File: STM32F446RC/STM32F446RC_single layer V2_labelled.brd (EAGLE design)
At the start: 80.2 x 29 mm, 75 parts, among them IC1 STM32F446RCT6

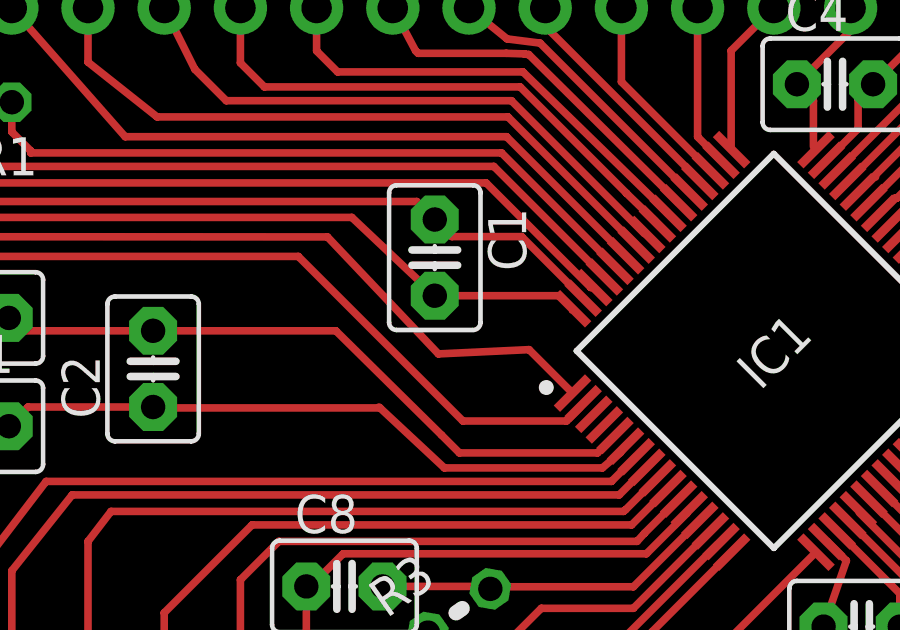
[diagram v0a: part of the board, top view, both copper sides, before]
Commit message: added final
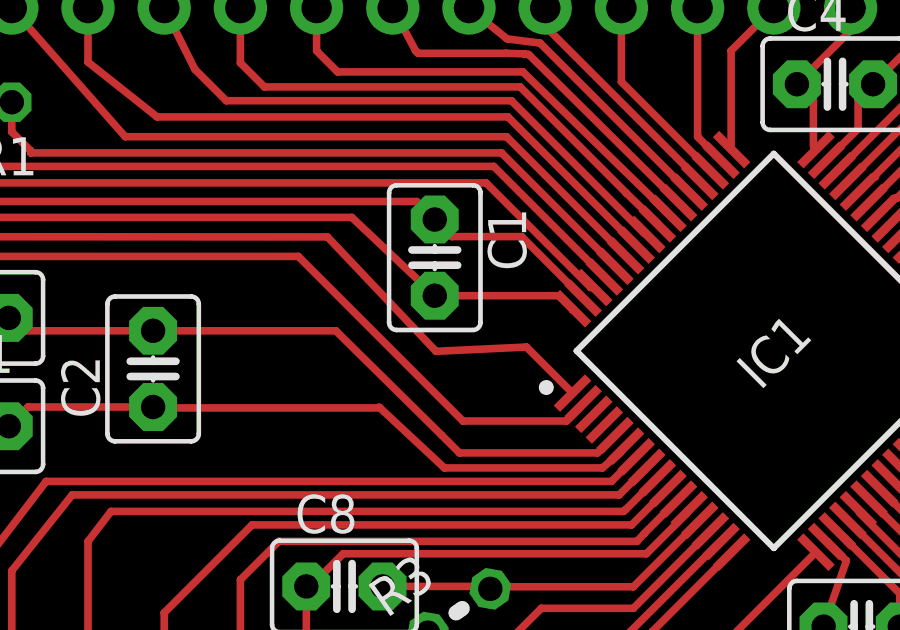
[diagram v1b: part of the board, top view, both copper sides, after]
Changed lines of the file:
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@@
 <layer number="16" name="Bottom" color="1" fill="1" visible="yes" active="yes"/>
 <layer number="17" name="Pads" color="2" fill="1" visible="yes" active="yes"/>
-<layer number="18" name="Vias" color="2" fill="1" visible="no" active="yes"/>
+<layer number="18" name="Vias" color="2" fill="1" visible="yes" active="yes"/>
 <layer number="19" name="Unrouted" color="6" fill="1" visible="yes" active="yes"/>
 <layer number="20" name="Dimension" color="24" fill="1" visible="yes" active="yes"/>
 <layer number="21" name="tPlace" color="7" fill="1" visible="yes" active="yes"/>
-<layer number="22" name="bPlace" color="7" fill="1" visible="no" active="yes"/>
+<layer number="22" name="bPlace" color="7" fill="1" visible="yes" active="yes"/>
 <layer number="23" name="tOrigins" color="15" fill="1" visible="yes" active="yes"/>
-<layer number="24" name="bOrigins" color="15" fill="1" visible="no" active="yes"/>
-<layer number="25" name="tNames" color="7" fill="1" visible="no" active="yes"/>
-<layer number="26" name="bNames" color="7" fill="1" visible="no" active="yes"/>
-<layer number="27" name="tValues" color="7" fill="1" visible="no" active="yes"/>
-<layer number="28" name="bValues" color="7" fill="1" visible="no" active="yes"/>
-<layer number="29" name="tStop" color="7" fill="3" visible="no" active="yes"/>
+<layer number="24" name="bOrigins" color="15" fill="1" visible="yes" active="yes"/>
+<layer number="25" name="tNames" color="7" fill="1" visible="yes" active="yes"/>
+<layer number="26" name="bNames" color="7" fill="1" visible="yes" active="yes"/>
+<layer number="27" name="tValues" color="7" fill="1" visible="yes" active="yes"/>
+<layer number="28" name="bValues" color="7" fill="1" visible="yes" active="yes"/>
+<layer number="29" name="tStop" color="7" fill="3" visible="yes" active="yes"/>
 <layer number="30" name="bStop" color="7" fill="6" visible="no" active="yes"/>
-<layer number="31" name="tCream" color="7" fill="4" visible="no" active="yes"/>
-<layer number="32" name="bCream" color="7" fill="5" visible="no" active="yes"/>
-<layer number="33" name="tFinish" color="6" fill="3" visible="no" active="yes"/>
-<layer number="34" name="bFinish" color="6" fill="6" visible="no" active="yes"/>
-<layer number="35" name="tGlue" color="7" fill="4" visible="no" active="yes"/>
-<layer number="36" name="bGlue" color="7" fill="5" visible="no" active="yes"/>
-<layer number="37" name="tTest" color="7" fill="1" visible="no" active="yes"/>
-<layer number="38" name="bTest" color="7" fill="1" visible="no" active="yes"/>
-<layer number="39" name="tKeepout" color="4" fill="11" visible="no" active="yes"/>
-<layer number="40" name="bKeepout" color="1" fill="11" visible="no" active="yes"/>
-<layer number="41" name="tRestrict" color="4" fill="10" visible="no" active="yes"/>
-<layer number="42" name="bRestrict" color="1" fill="10" visible="no" active="yes"/>
-<layer number="43" name="vRestrict" color="2" fill="10" visible="no" active="yes"/>
-<layer number="44" name="Drills" color="7" fill="1" visible="no" active="yes"/>
-<layer number="45" name="Holes" color="7" fill="1" visible="no" active="yes"/>
-<layer number="46" name="Milling" color="3" fill="1" visible="no" active="yes"/>
-<layer number="47" name="Measures" color="7" fill="1" visible="no" active="yes"/>
+<layer number="31" name="tCream" color="7" fill="4" visible="yes" active="yes"/>
+<layer number="32" name="bCream" color="7" fill="5" visible="yes" active="yes"/>
+<layer number="33" name="tFinish" color="6" fill="3" visible="yes" active="yes"/>
+<layer number="34" name="bFinish" color="6" fill="6" visible="yes" active="yes"/>
+<layer number="35" name="tGlue" color="7" fill="4" visible="yes" active="yes"/>
+<layer number="36" name="bGlue" color="7" fill="5" visible="yes" active="yes"/>
+<layer number="37" name="tTest" color="7" fill="1" visible="yes" active="yes"/>
+<layer number="38" name="bTest" color="7" fill="1" visible="yes" active="yes"/>
+<layer number="39" name="tKeepout" color="4" fill="11" visible="yes" active="yes"/>
+<layer number="40" name="bKeepout" color="1" fill="11" visible="yes" active="yes"/>
+<layer number="41" name="tRestrict" color="4" fill="10" visible="yes" active="yes"/>
+<layer number="42" name="bRestrict" color="1" fill="10" visible="yes" active="yes"/>
+<layer number="43" name="vRestrict" color="2" fill="10" visible="yes" active="yes"/>
+<layer number="44" name="Drills" color="7" fill="1" visible="yes" active="yes"/>
+<layer number="45" name="Holes" color="7" fill="1" visible="yes" active="yes"/>
+<layer number="46" name="Milling" color="3" fill="1" visible="yes" active="yes"/>
+<layer number="47" name="Measures" color="7" fill="1" visible="yes" active="yes"/>
 <layer number="48" name="Document" color="7" fill="1" visible="yes" active="yes"/>
-<layer number="49" name="Reference" color="7" fill="1" visible="no" active="yes"/>
+<layer number="49" name="Reference" color="7" fill="1" visible="yes" active="yes"/>
 <layer number="50" name="dxf" color="7" fill="1" visible="no" active="no"/>
-<layer number="51" name="tDocu" color="7" fill="1" visible="no" active="yes"/>
+<layer number="51" name="tDocu" color="7" fill="1" visible="yes" active="yes"/>
 <layer number="52" name="bDocu" color="7" fill="1" visible="yes" active="yes"/>
 <layer number="53" name="tGND_GNDA" color="7" fill="1" visible="no" active="no"/>
@@
 <layer number="221" name="221bmp" color="7" fill="1" visible="yes" active="yes"/>
 <layer number="222" name="222bmp" color="7" fill="1" visible="yes" active="yes"/>
-<layer number="223" name="223bmp" color="7" fill="1" visible="no" active="yes"/>
-<layer number="224" name="224bmp" color="7" fill="1" visible="no" active="yes"/>
-<layer number="250" name="Descript" color="7" fill="1" visible="no" active="yes"/>
-<layer number="251" name="SMDround" color="7" fill="1" visible="no" active="yes"/>
-<layer number="254" name="cooling" color="7" fill="1" visible="no" active="yes"/>
+<layer number="223" name="223bmp" color="7" fill="1" visible="yes" active="yes"/>
+<layer number="224" name="224bmp" color="7" fill="1" visible="yes" active="yes"/>
+<layer number="250" name="Descript" color="7" fill="1" visible="yes" active="yes"/>
+<layer number="251" name="SMDround" color="7" fill="1" visible="yes" active="yes"/>
+<layer number="254" name="cooling" color="7" fill="1" visible="yes" active="yes"/>
 </layers>
 <board>
@@
 <contactref element="IC1" pad="1"/>
 <wire x1="33.41096875" y1="12.99426875" x2="33.3636" y2="13.13" width="0.1524" layer="1"/>
-<wire x1="33.41096875" y1="12.99426875" x2="31.962575" y2="14.4426625" width="0.254" layer="1"/>
+<wire x1="33.41096875" y1="12.99426875" x2="31.876096875" y2="14.529140625" width="0.254" layer="1"/>
 <wire x1="5.950053125" y1="18.209309375" x2="4.56" y2="18.21" width="0.254" layer="1"/>
 <wire x1="25.2420125" y1="18.199728125" x2="5.950053125" y2="18.209309375" width="0.254" layer="1"/>
-<wire x1="28.93999375" y1="14.3" x2="25.2420125" y2="18.199728125" width="0.254" layer="1"/>
-<wire x1="31.962575" y1="14.4426625" x2="28.93999375" y2="14.3" width="0.254" layer="1"/>
+<wire x1="28.857796875" y1="14.38668125" x2="25.2420125" y2="18.199728125" width="0.254" layer="1"/>
+<wire x1="31.876096875" y1="14.529140625" x2="28.857796875" y2="14.38668125" width="0.254" layer="1"/>
 <wire x1="4.56" y1="18.21" x2="4.56" y2="2.97" width="0.254" layer="1"/>
 </signal>
